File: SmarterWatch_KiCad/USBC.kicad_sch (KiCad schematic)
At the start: 5 parts, among them J5 CX70M-24P1

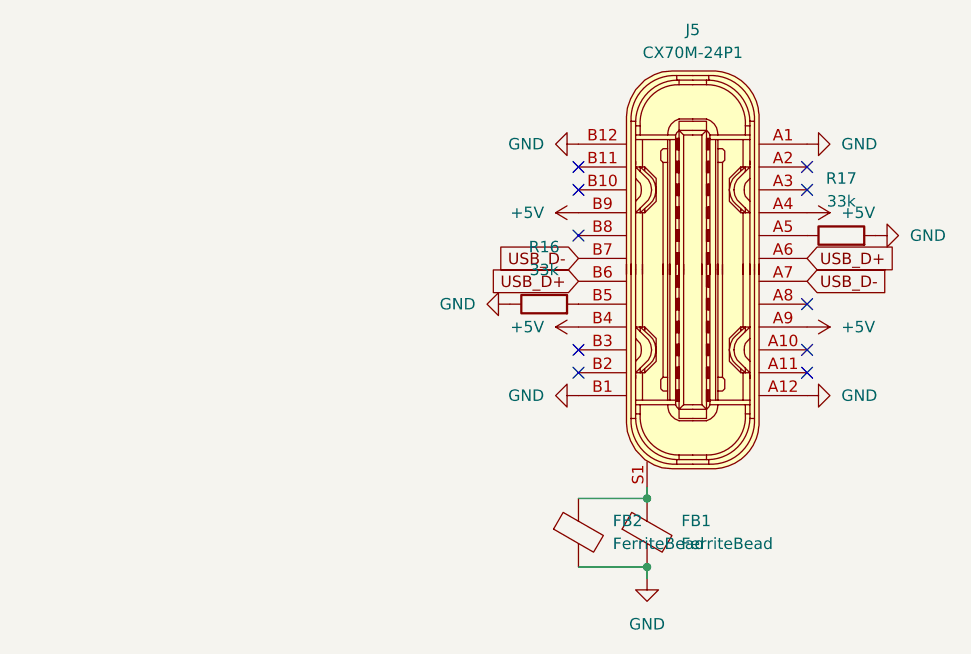
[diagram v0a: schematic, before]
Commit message: update
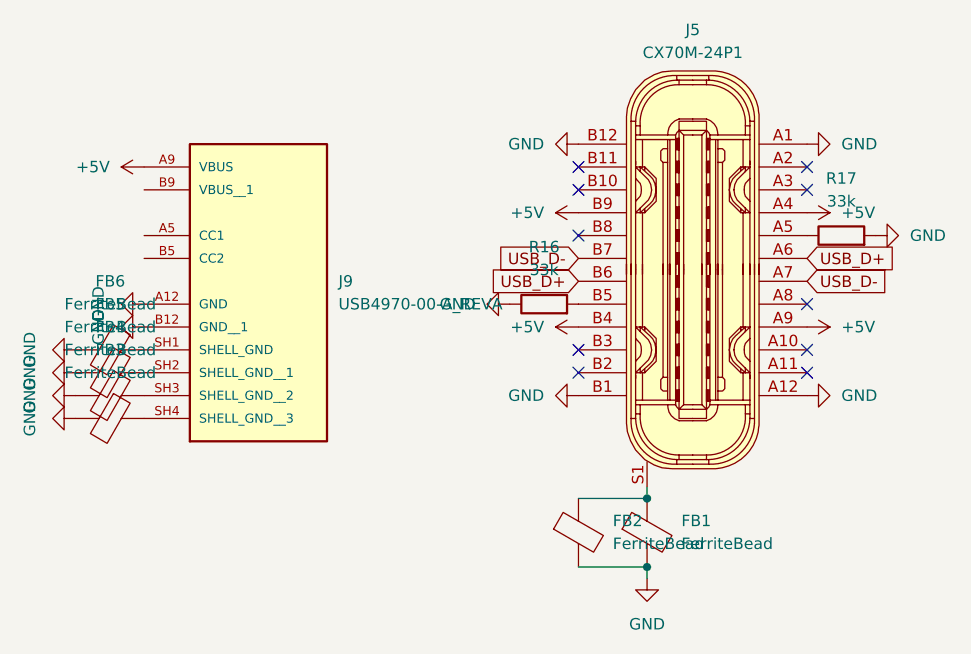
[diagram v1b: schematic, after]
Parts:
- added FB3, FB4, FB5, FB6: FerriteBead, Resistor_SMD:R_0402_1005Metric, symbol Device:FerriteBead
- added J9: USB4970-00-A_REVA, USB4970-00-A_REVA:GCT_USB4970-00-A_REVA, symbol USB4970-00-A_REVA:USB4970-00-A_REVA
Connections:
- net +5V: now also J9.A9 (VBUS)
- net GND: now also FB3.2, FB4.2, FB5.2, FB6.2, J9.A12 (GND), J9.B12 (GND__1)
- new net: FB3.1, J9.SH4 (SHELL_GND__3)
- new net: FB6.1, J9.SH1 (SHELL_GND)
- new net: FB5.1, J9.SH2 (SHELL_GND__1)
- new net: FB4.1, J9.SH3 (SHELL_GND__2)
